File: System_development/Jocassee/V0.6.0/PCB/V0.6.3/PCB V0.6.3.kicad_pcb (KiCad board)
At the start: 2 copper layers, 33 x 122.5 mm, 32 parts, among them J1 TDS PRB, J2 Temp, J3 BAT, J4 TRBDT, J5 CHRG, J6 Conn_Coaxial_Small, P1 SD card socket, Q1 2N2222A, U1 NRF24L01+PA+LNA, U2 ProMicro, U3 EZO_PH, U4 EZO_TDS, U5 DC-DC STPDN LM2596, U6 HX-2S-JH10, U7 BOB-12009, level shifter, U8 AMS1117 3.3v

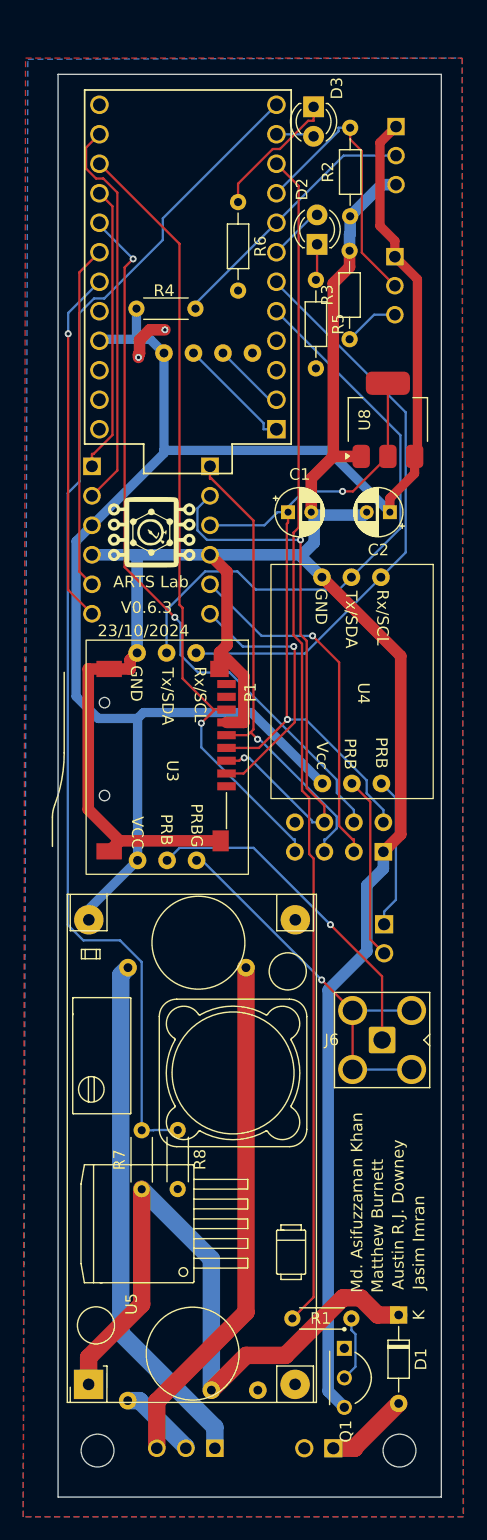
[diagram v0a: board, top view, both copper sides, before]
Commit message: PCB refined
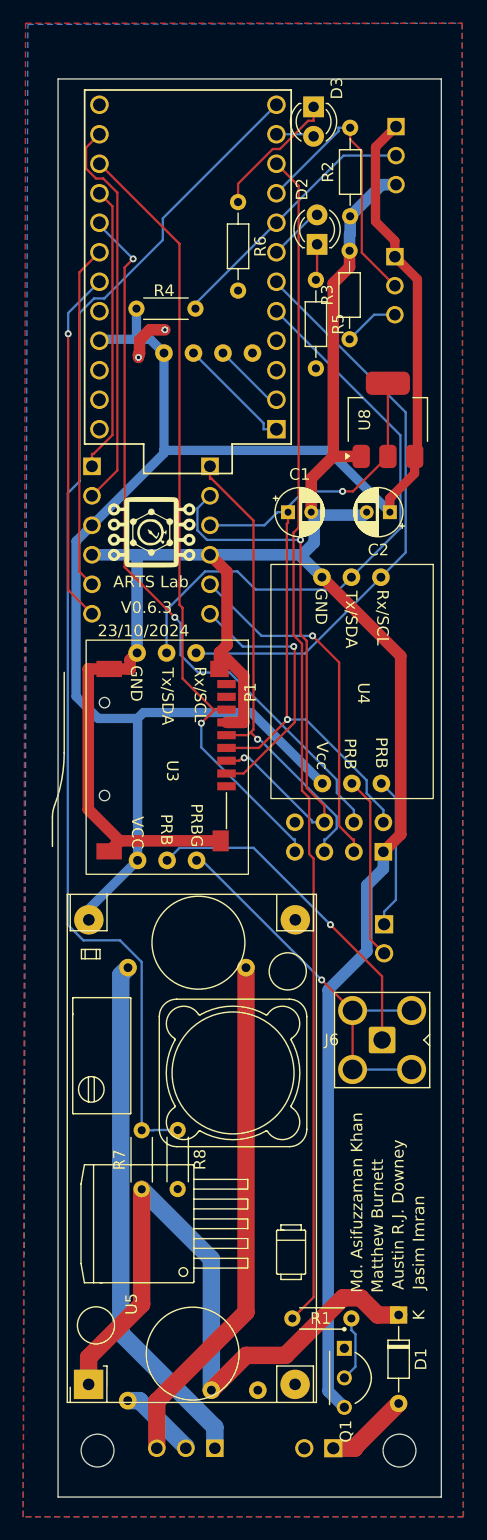
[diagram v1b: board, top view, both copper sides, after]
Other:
- board size 33 x 122.5 mm -> 33 x 122.1 mm
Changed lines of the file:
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@@
 		(fp_arc
 			(start 13.181636 16.183217)
-			(mid 13.252317 16.21252)
+			(mid 13.252353 16.212514)
 			(end 13.281636 16.283217)
 			(stroke
@@
 		(fp_arc
 			(start 23.847611 17.472062)
-			(mid 23.907831 17.428018)
+			(mid 23.907846 17.427997)
 			(end 23.981783 17.437976)
 			(stroke
@@
 		(fp_arc
 			(start 9.581636 18.683217)
-			(mid 9.510896 18.653941)
+			(mid 9.510931 18.653935)
 			(end 9.481636 18.583217)
 			(stroke
@@
 	)
 	(gr_rect
-		(start 79.6 64.5)
+		(start 79.6 64.9)
 		(end 112.6 187)
 		(stroke
@@
 	)
 	(segment
-		(start 110.5437 82.1437)
-		(end 108.6 80.2)
+		(start 106.934 70.766)
+		(end 108.7 69)
 		(width 0.8)
 		(layer "F.Cu")
@@
 	)
 	(segment
-		(start 108.6 78.8443)
-		(end 107.3167 77.561)
+		(start 110.5437 82.1437)
+		(end 108.6 80.2)
 		(width 0.8)
 		(layer "F.Cu")
@@
 	)
 	(segment
-		(start 108.6 80.2)
-		(end 108.6 78.8443)
+		(start 108.6 78.8443)
+		(end 106.934 77.1783)
 		(width 0.8)
 		(layer "F.Cu")
@@
 	)
 	(segment
-		(start 107.3167 77.561)
-		(end 107.3167 70.3833)
+		(start 106.934 77.1783)
+		(end 106.934 70.766)
 		(width 0.8)
 		(layer "F.Cu")
@@
 	)
 	(segment
-		(start 107.3167 70.3833)
-		(end 108.7 69)
+		(start 108.6 80.2)
+		(end 108.6 78.8443)
 		(width 0.8)
 		(layer "F.Cu")
@@
 		(polygon
 			(pts
-				(xy 76.8 63.1) (xy 114.4 63.1) (xy 114.5 188.7) (xy 76.6 188.7)
+				(xy 76.8 60.1) (xy 114.4 60.1) (xy 114.5 188.7) (xy 76.6 188.7)
 			)
 		)
@@
 		(polygon
 			(pts
-				(xy 77 63.2) (xy 114.4 63.1) (xy 114.5 188.7) (xy 76.6 188.7)
+				(xy 77 60.2) (xy 114.4 60.1) (xy 114.5 188.7) (xy 76.6 188.7)
 			)
 		)
